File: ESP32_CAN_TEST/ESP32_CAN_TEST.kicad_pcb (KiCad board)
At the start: 2 copper layers, 45.7 x 45.7 mm, 45 parts, among them J1 XT60, J2 Encoder_1, J3 Molex_2x2, J4 Encoder2, J5 Molex_2x2, J6 UART, J7 GH1.25, SW1 EN, SW2 EN, U1 AMS1117, U2 ESP32-WROOM-32, U3 MP2451, U4 TJA1051T, U5 TJA1051T

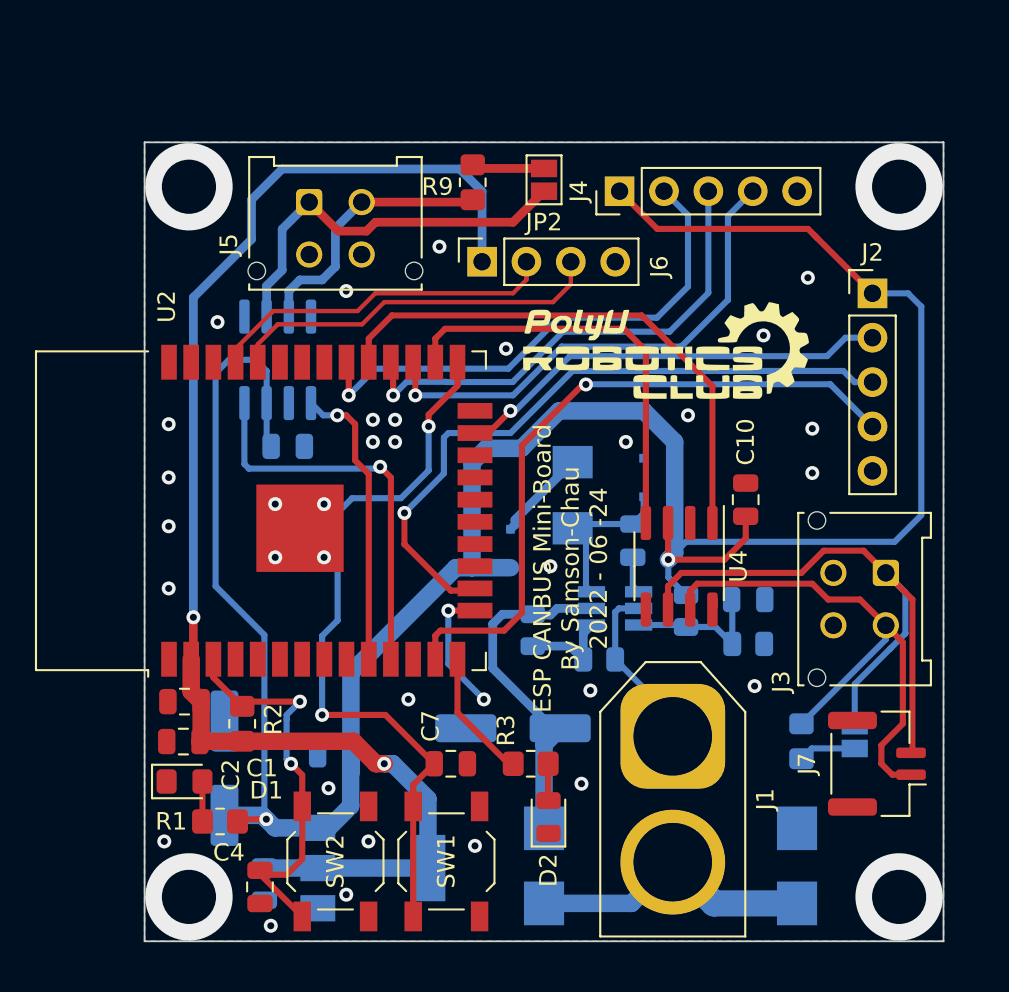
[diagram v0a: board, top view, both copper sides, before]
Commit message: sad
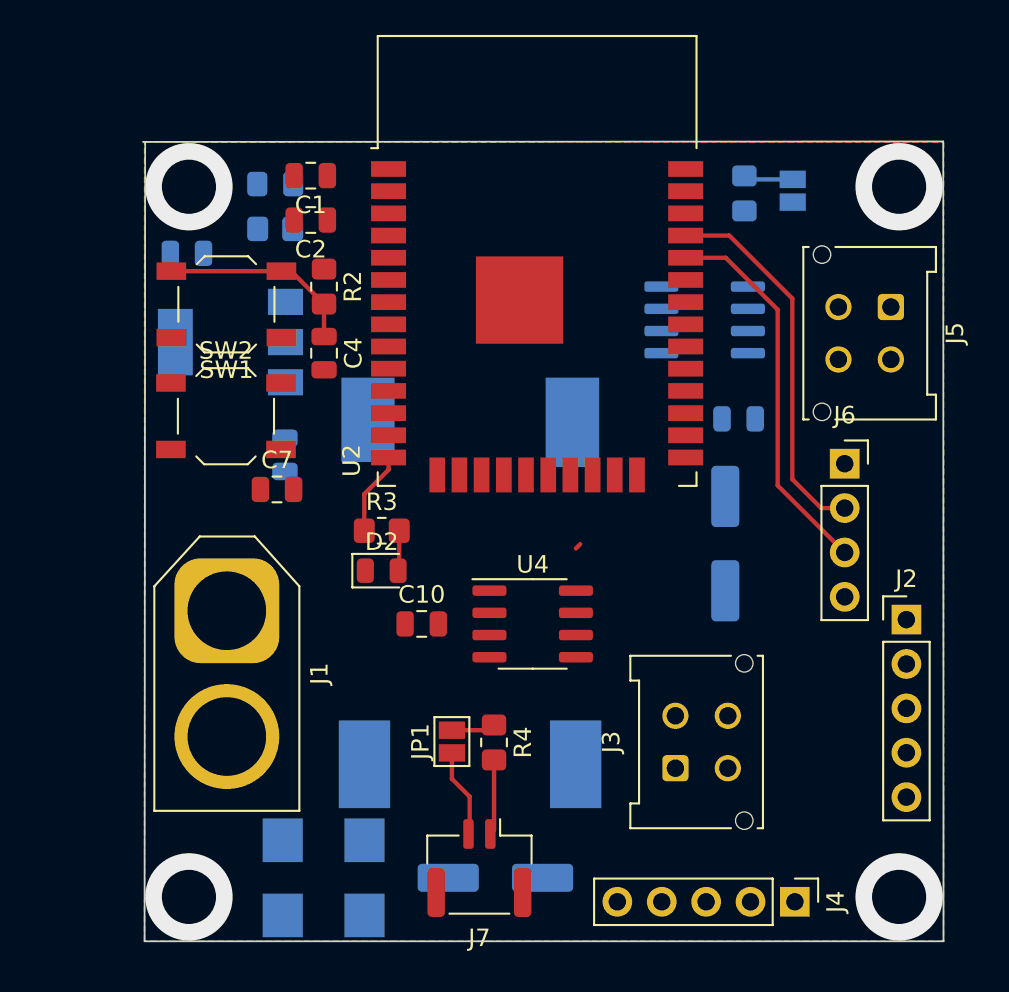
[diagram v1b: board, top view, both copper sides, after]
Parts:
- removed C11: 100pF, Capacitor_SMD:C_0805_2012Metric
- removed C8: 100nF, Capacitor_SMD:C_0805_2012Metric
- removed D5, D6: S4, Diode_SMD:D_SOD-323F
- removed G***: LOGO, PolyuRobotics:Club_logo
- removed L1: 3.3uH, Inductor_SMD:L_Vishay_IHLP-1616
- removed R5: 27K, Resistor_SMD:R_0805_2012Metric
- removed R6: 22k, Resistor_SMD:R_0805_2012Metric
- removed R7: 124K, Resistor_SMD:R_0805_2012Metric
- removed R8: 2K2, Resistor_SMD:R_0805_2012Metric
- D1, JP2, R1, R9: moved to B.Cu
- JP1, R4: moved to F.Cu
- U3: value MP2451 -> MP1584; footprint Package_TO_SOT_SMD:SOT-23-6_Handsoldering -> PolyuRobotics:DC-DC-mp1584_module
- moved J4 41.9 mm to (144.0, 119.8), turned to -90 degrees
- moved C5 36.3 mm to (109.2, 82.7), turned to 0 degrees
- moved D1 34.6 mm to (114.3, 78.7), turned to 180 degrees
- moved R1 34.1 mm to (114.3, 81.3)
- moved J5 33.8 mm to (149.5, 85.8), turned to -90 degrees
- moved C1 33.2 mm to (116.3, 78.2)
- moved SW1 32.5 mm to (111.5, 85.6), turned to 180 degrees
- moved C9 31.4 mm to (140.1, 99.3), turned to -90 degrees
- moved U1 31.2 mm to (111.7, 87.8), turned to 180 degrees
- moved C4 30.8 mm to (117.1, 88.4)
- moved D3 29.4 mm to (114.7, 118.4)
- moved C2 28.5 mm to (116.3, 80.8)
- moved SW2 28.4 mm to (111.5, 92.0), turned to 0 degrees
- moved J1 26.5 mm to (111.5, 103.1)
- moved C12 25.8 mm to (140.8, 92.2)
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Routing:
- net +5V: track 149.8 -> 0.00 mm, vias 2 -> 0
- net +3V3: track 79.1 -> 0.00 mm, vias 2 -> 0
- net Net-(C7-Pad2): track 41.8 -> 0.35 mm, vias 2 -> 0
- net /IO14: track 38.9 -> 0.00 mm, vias 1 -> 0
- net /IO13: track 38.6 -> 0.00 mm, vias 1 -> 0
- net /CANH+: track 36.5 -> 5.09 mm
- net /CAN_TX: track 31.1 -> 0.00 mm
- net /IO18: track 30.0 -> 0.00 mm, vias 1 -> 0
- net /IO16: track 28.9 -> 0.00 mm, vias 1 -> 0
- net /IO17: track 28.2 -> 0.00 mm, vias 1 -> 0
- net /CANL-: track 31.8 -> 4.33 mm
- net /IO15: track 25.0 -> 0.00 mm, vias 1 -> 0
- net /CAN_RX: track 24.0 -> 0.00 mm
- net /CAN2_RX: track 22.7 -> 0.00 mm, vias 1 -> 0
- net /CAN2H+: track 22.6 -> 0.00 mm
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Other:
- board size 45.7 x 45.7 mm -> 45.8 x 45.8 mm
- board text removed: "ESP CANBUS Mini-Board By Samson-Chau 2022 - 06 -24"
